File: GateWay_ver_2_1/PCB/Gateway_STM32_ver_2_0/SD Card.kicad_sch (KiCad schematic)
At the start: 2 parts, among them J9 Micro_SD_Card

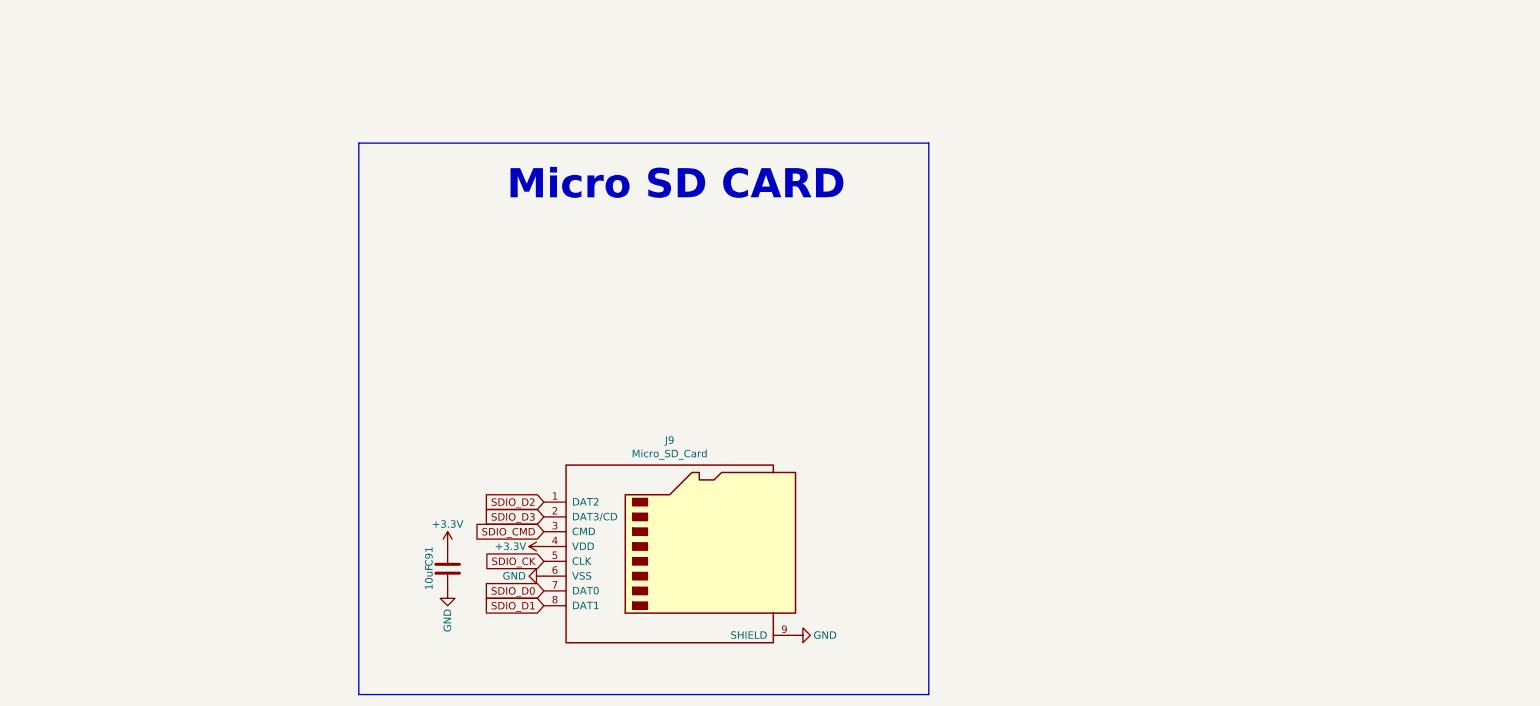
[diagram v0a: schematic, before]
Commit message: 1
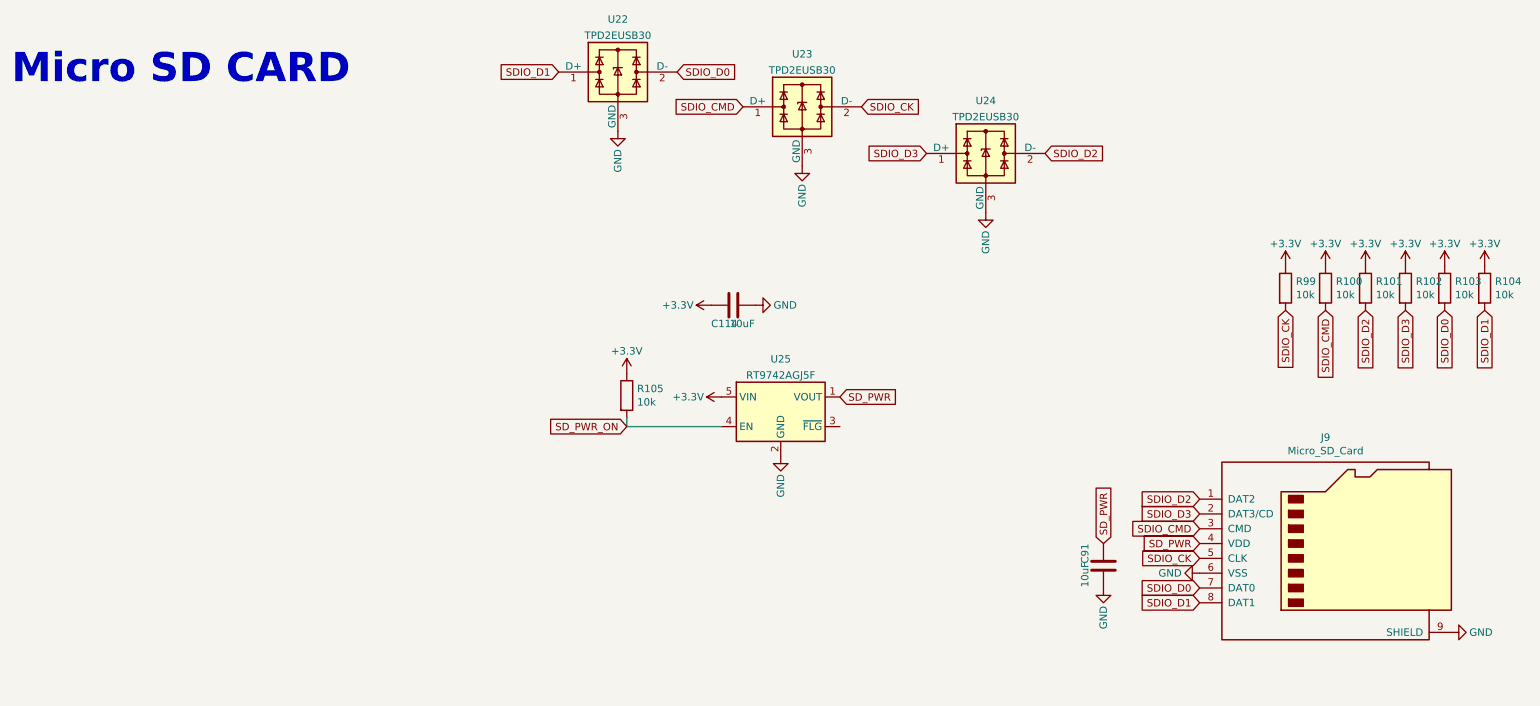
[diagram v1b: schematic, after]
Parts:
- added C114: 10uF, Capacitor_SMD:C_0805_2012Metric, symbol Device:C
- added R100, R101, R102, R103, R104, R105, R99: 10k, Resistor_SMD:R_0603_1608Metric, symbol Device:R
- added U22, U23, U24: TPD2EUSB30, Package_TO_SOT_SMD:Texas_DRT-3, symbol Power_Protection:TPD2EUSB30
- added U25: RT9742AGJ5F, Package_TO_SOT_SMD:TSOT-23-5, symbol Power_Management:RT9742AGJ5F
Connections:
- net +3V3: now also C114.2, R100.1, R101.1, R102.1, R103.1, R104.1, R105.1, R99.1, U25.5 (VIN); no longer C91.2, J9.4 (VDD)
- net GND: now also C114.1, U22.3 (GND), U23.3 (GND), U24.3 (GND), U25.2 (GND)
- net SDIO_CK: now also R99.2, U23.2 (D-)
- net SDIO_CMD: now also R100.2, U23.1 (D+)
- net SDIO_D0: now also R103.2, U22.2 (D-)
- net SDIO_D1: now also R104.2, U22.1 (D+)
- net SDIO_D2: now also R101.2, U24.2 (D-)
- net SDIO_D3: now also R102.2, U24.1 (D+)
- new net SD_PWR: C91.2, J9.4 (VDD), U25.1 (VOUT)
- new net SD_PWR_ON: R105.2, U25.4 (EN)
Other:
- moved on the sheet: C91, J9
